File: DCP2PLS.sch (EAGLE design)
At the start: 2 parts, among them CON4 CON-6P, CON6 PINHEAD_1X06-2.54

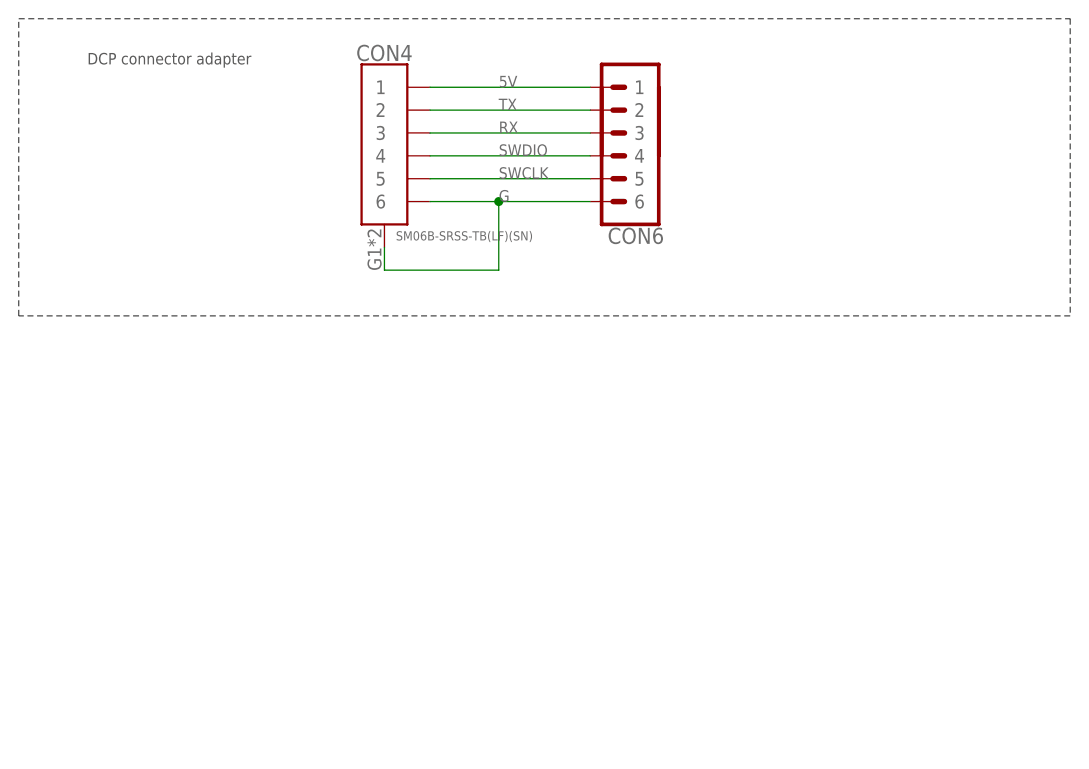
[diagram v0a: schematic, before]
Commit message: updates
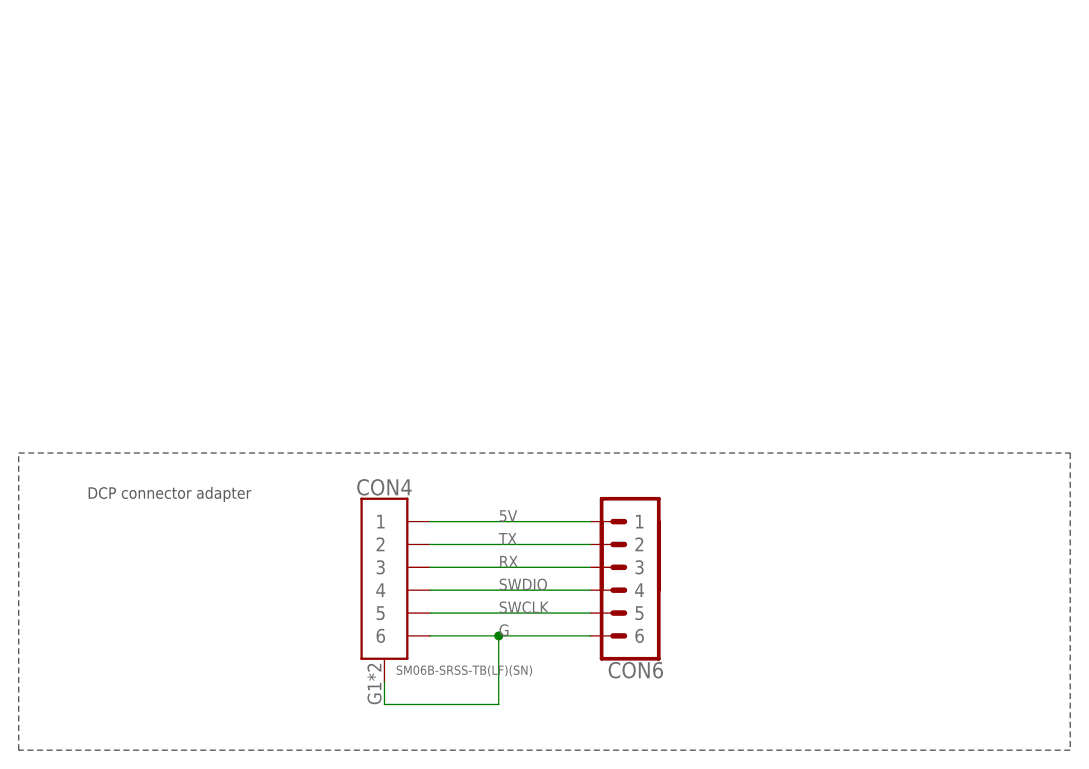
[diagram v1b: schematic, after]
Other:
- moved on the sheet: CON4, CON6
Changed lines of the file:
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@@
 <sheet>
 <plain>
-<wire x1="7.62" y1="149.86" x2="124.46" y2="149.86" width="0.1524" layer="97" style="shortdash"/>
-<wire x1="124.46" y1="149.86" x2="124.46" y2="116.84" width="0.1524" layer="97" style="shortdash"/>
-<wire x1="124.46" y1="116.84" x2="7.62" y2="116.84" width="0.1524" layer="97" style="shortdash"/>
-<wire x1="7.62" y1="116.84" x2="7.62" y2="149.86" width="0.1524" layer="97" style="shortdash"/>
-<text x="15.24" y="144.78" size="1.27" layer="97">DCP connector adapter</text>
+<wire x1="7.62" y1="101.6" x2="124.46" y2="101.6" width="0.1524" layer="97" style="shortdash"/>
+<wire x1="124.46" y1="101.6" x2="124.46" y2="68.58" width="0.1524" layer="97" style="shortdash"/>
+<wire x1="124.46" y1="68.58" x2="7.62" y2="68.58" width="0.1524" layer="97" style="shortdash"/>
+<wire x1="7.62" y1="68.58" x2="7.62" y2="101.6" width="0.1524" layer="97" style="shortdash"/>
+<text x="15.24" y="96.52" size="1.27" layer="97">DCP connector adapter</text>
 </plain>
 <instances>
-<instance part="CON4" gate="P" x="45.72" y="127"/>
+<instance part="CON4" gate="P" x="45.72" y="78.74"/>
 <instance part="FRAME1" gate="G$1" x="0" y="0"/>
-<instance part="CON6" gate="G$1" x="78.74" y="144.78" rot="R180"/>
+<instance part="CON6" gate="G$1" x="78.74" y="96.52" rot="R180"/>
 </instances>
 <busses>
@@
 <segment>
 <pinref part="CON4" gate="P" pin="1"/>
-<wire x1="53.34" y1="142.24" x2="71.12" y2="142.24" width="0.1524" layer="91"/>
-<label x="60.96" y="142.24" size="1.27" layer="95"/>
+<wire x1="53.34" y1="93.98" x2="71.12" y2="93.98" width="0.1524" layer="91"/>
+<label x="60.96" y="93.98" size="1.27" layer="95"/>
 <pinref part="CON6" gate="G$1" pin="1"/>
 </segment>
@@
 <segment>
 <pinref part="CON4" gate="P" pin="2"/>
-<wire x1="53.34" y1="139.7" x2="71.12" y2="139.7" width="0.1524" layer="91"/>
-<label x="60.96" y="139.7" size="1.27" layer="95"/>
+<wire x1="53.34" y1="91.44" x2="71.12" y2="91.44" width="0.1524" layer="91"/>
+<label x="60.96" y="91.44" size="1.27" layer="95"/>
 <pinref part="CON6" gate="G$1" pin="2"/>
 </segment>
@@
 <segment>
 <pinref part="CON4" gate="P" pin="3"/>
-<wire x1="53.34" y1="137.16" x2="71.12" y2="137.16" width="0.1524" layer="91"/>
-<label x="60.96" y="137.16" size="1.27" layer="95"/>
+<wire x1="53.34" y1="88.9" x2="71.12" y2="88.9" width="0.1524" layer="91"/>
+<label x="60.96" y="88.9" size="1.27" layer="95"/>
 <pinref part="CON6" gate="G$1" pin="3"/>
 </segment>
@@
 <segment>
 <pinref part="CON4" gate="P" pin="4"/>
-<wire x1="53.34" y1="134.62" x2="71.12" y2="134.62" width="0.1524" layer="91"/>
-<label x="60.96" y="134.62" size="1.27" layer="95"/>
+<wire x1="53.34" y1="86.36" x2="71.12" y2="86.36" width="0.1524" layer="91"/>
+<label x="60.96" y="86.36" size="1.27" layer="95"/>
 <pinref part="CON6" gate="G$1" pin="4"/>
 </segment>
@@
 <segment>
 <pinref part="CON4" gate="P" pin="5"/>
-<wire x1="53.34" y1="132.08" x2="71.12" y2="132.08" width="0.1524" layer="91"/>
-<label x="60.96" y="132.08" size="1.27" layer="95"/>
+<wire x1="53.34" y1="83.82" x2="71.12" y2="83.82" width="0.1524" layer="91"/>
+<label x="60.96" y="83.82" size="1.27" layer="95"/>
 <pinref part="CON6" gate="G$1" pin="5"/>
 </segment>
@@
 <segment>
 <pinref part="CON4" gate="P" pin="6"/>
-<wire x1="53.34" y1="129.54" x2="60.96" y2="129.54" width="0.1524" layer="91"/>
-<label x="60.96" y="129.54" size="1.27" layer="95"/>
+<wire x1="53.34" y1="81.28" x2="60.96" y2="81.28" width="0.1524" layer="91"/>
+<label x="60.96" y="81.28" size="1.27" layer="95"/>
 <pinref part="CON6" gate="G$1" pin="6"/>
 <pinref part="CON4" gate="P" pin="G1"/>
-<wire x1="60.96" y1="129.54" x2="71.12" y2="129.54" width="0.1524" layer="91"/>
-<wire x1="48.26" y1="124.46" x2="48.26" y2="121.92" width="0.1524" layer="91"/>
-<wire x1="48.26" y1="121.92" x2="60.96" y2="121.92" width="0.1524" layer="91"/>
-<wire x1="60.96" y1="121.92" x2="60.96" y2="129.54" width="0.1524" layer="91"/>
-<junction x="60.96" y="129.54"/>
+<wire x1="60.96" y1="81.28" x2="71.12" y2="81.28" width="0.1524" layer="91"/>
+<wire x1="48.26" y1="76.2" x2="48.26" y2="73.66" width="0.1524" layer="91"/>
+<wire x1="48.26" y1="73.66" x2="60.96" y2="73.66" width="0.1524" layer="91"/>
+<wire x1="60.96" y1="73.66" x2="60.96" y2="81.28" width="0.1524" layer="91"/>
+<junction x="60.96" y="81.28"/>
 </segment>
 </net>
